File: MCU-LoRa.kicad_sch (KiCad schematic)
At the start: 8 parts, among them J7 castellated_1x08_P2.54, J8 castellated_1x08_P2.54

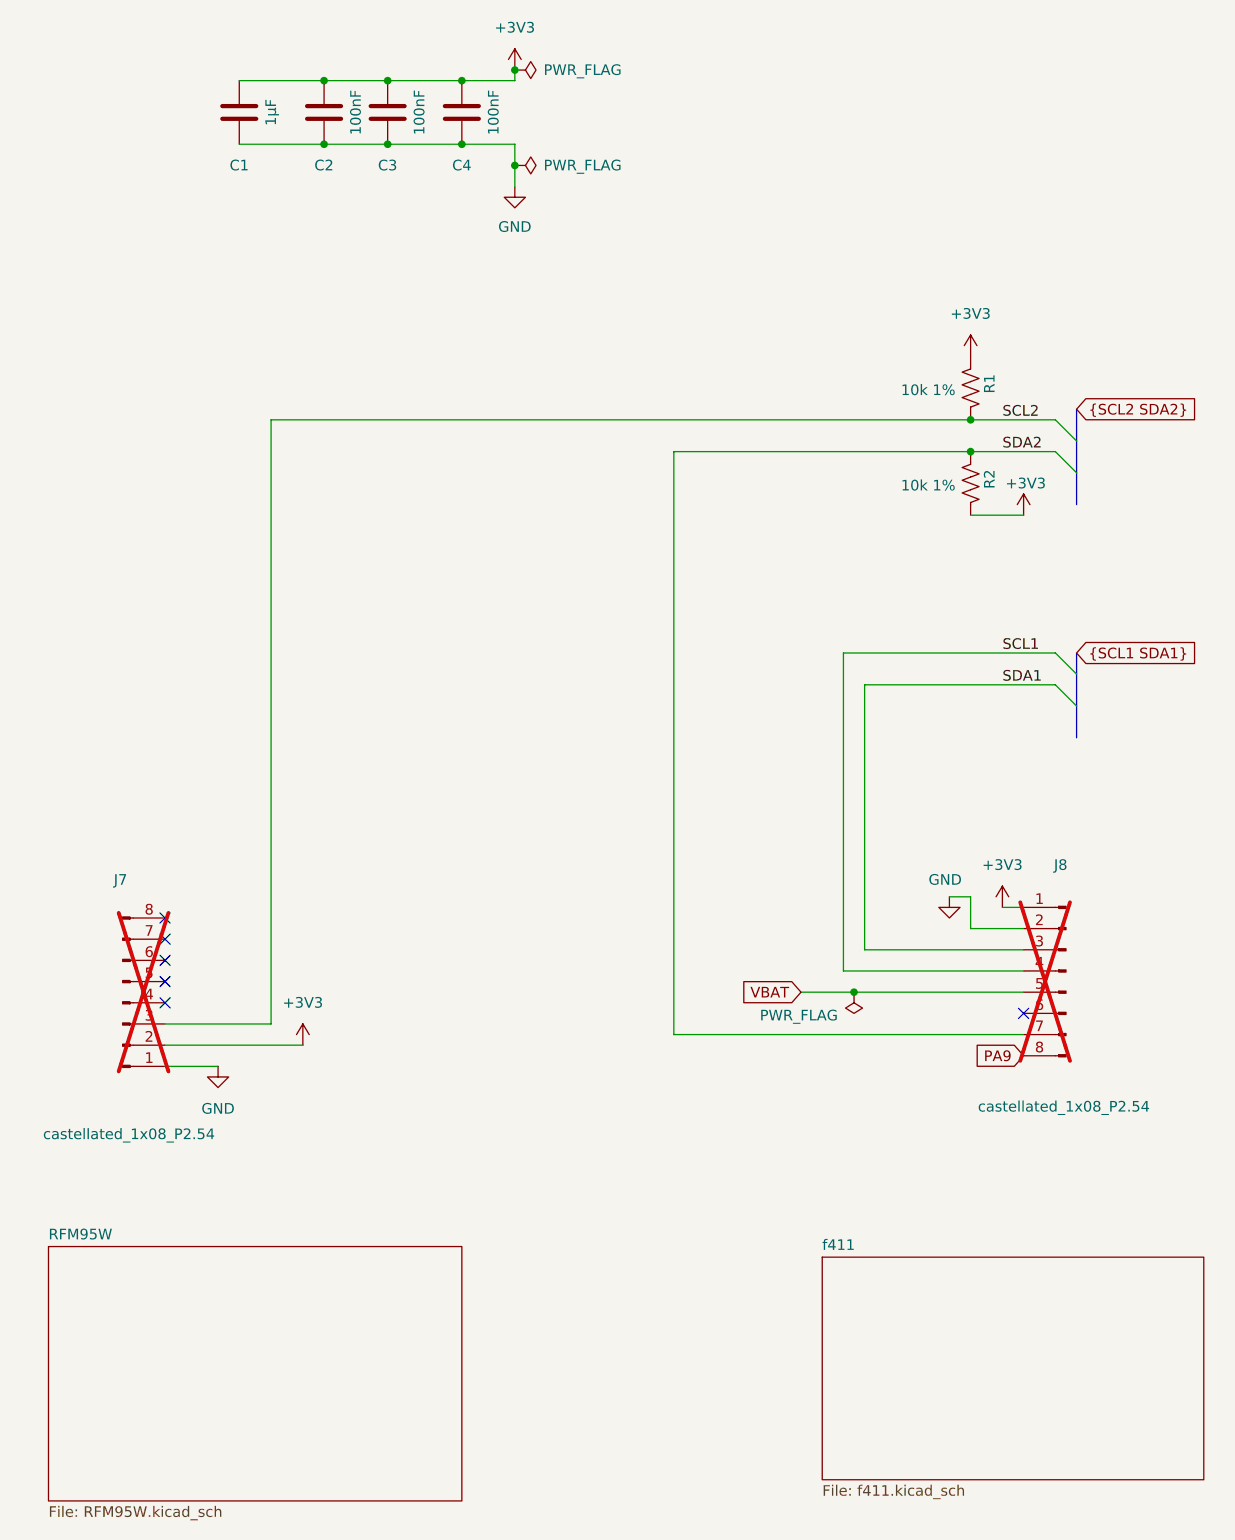
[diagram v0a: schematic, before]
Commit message: ongoing
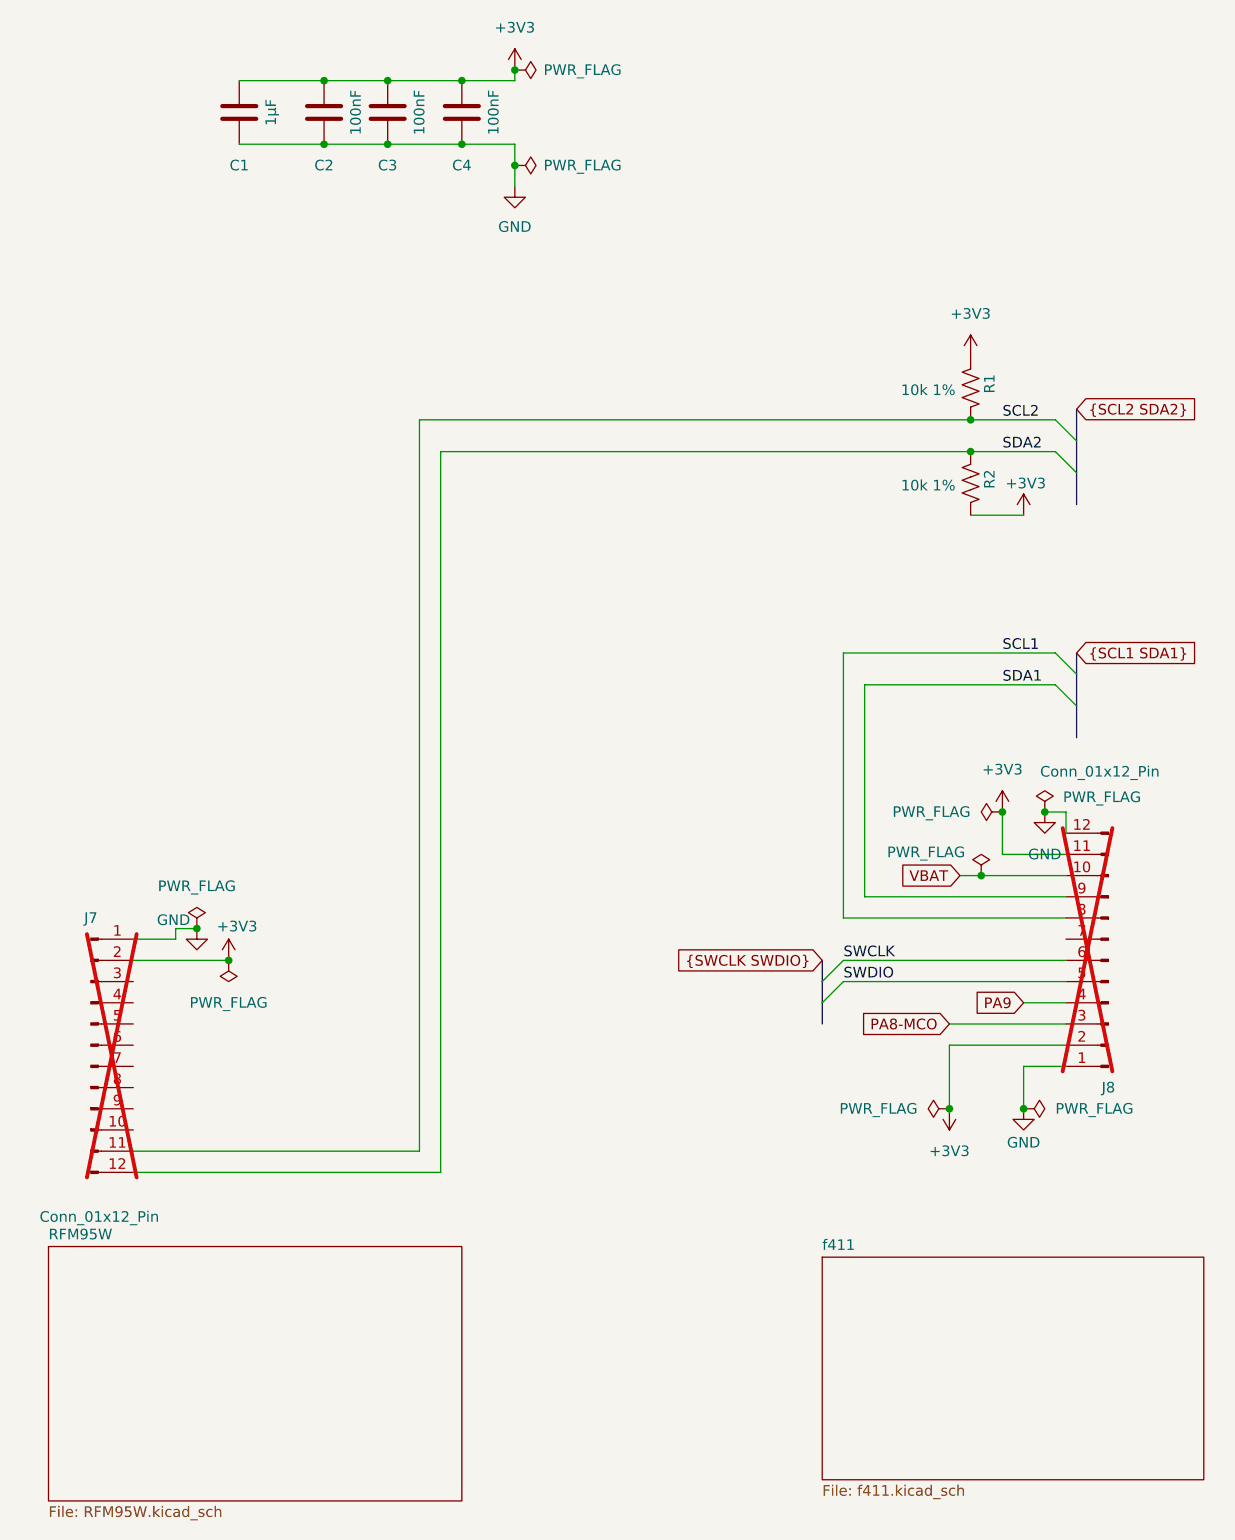
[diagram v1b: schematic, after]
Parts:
- J7, J8: value castellated_1x08_P2.54 -> Conn_01x12_Pin; footprint ProjectLib:castellated_1x08_P2.54mm -> ProjectLib:Castellated_Header_1x12_P2.00mm_Vertical; symbol ProjectLib:Conn_01x08_Pin -> ProjectLib:Conn_01x12_Pin
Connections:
- net +3V3: now also J8.11 (Pin_11), J8.2 (Pin_2); no longer J8.1 (Pin_1)
- net GND: now also J8.1 (Pin_1), J8.12 (Pin_12); no longer J8.2 (Pin_2)
- net PA9: now also J8.4 (Pin_4); no longer J8.8 (Pin_8)
- net SCL1: now also J8.8 (Pin_8); no longer J8.4 (Pin_4)
- net SCL2: now also J7.11 (Pin_11); no longer J7.3 (Pin_3)
- net SDA1: now also J8.9 (Pin_9); no longer J8.3 (Pin_3)
- net SDA2: now also J7.12 (Pin_12); no longer J8.7 (Pin_7)
- net VBAT: now also J8.10 (Pin_10); no longer J8.5 (Pin_5)
- net SWCLK: now reaches J8.6 (Pin_6)
- new net PA8-MCO: J8.3 (Pin_3)
- new net SWDIO: J8.5 (Pin_5)
- no-connect marks 6 -> 0
